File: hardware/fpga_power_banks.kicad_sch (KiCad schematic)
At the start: 0 parts

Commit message: update FPGA banks schematics
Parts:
- added U4: MPFS025T-FCVG484E, MPFS250T/MPFS160T/MPFS095T/MPFS025T-FCVG484_MCH, symbol payload-sym:MPFS025T-FCVG484E

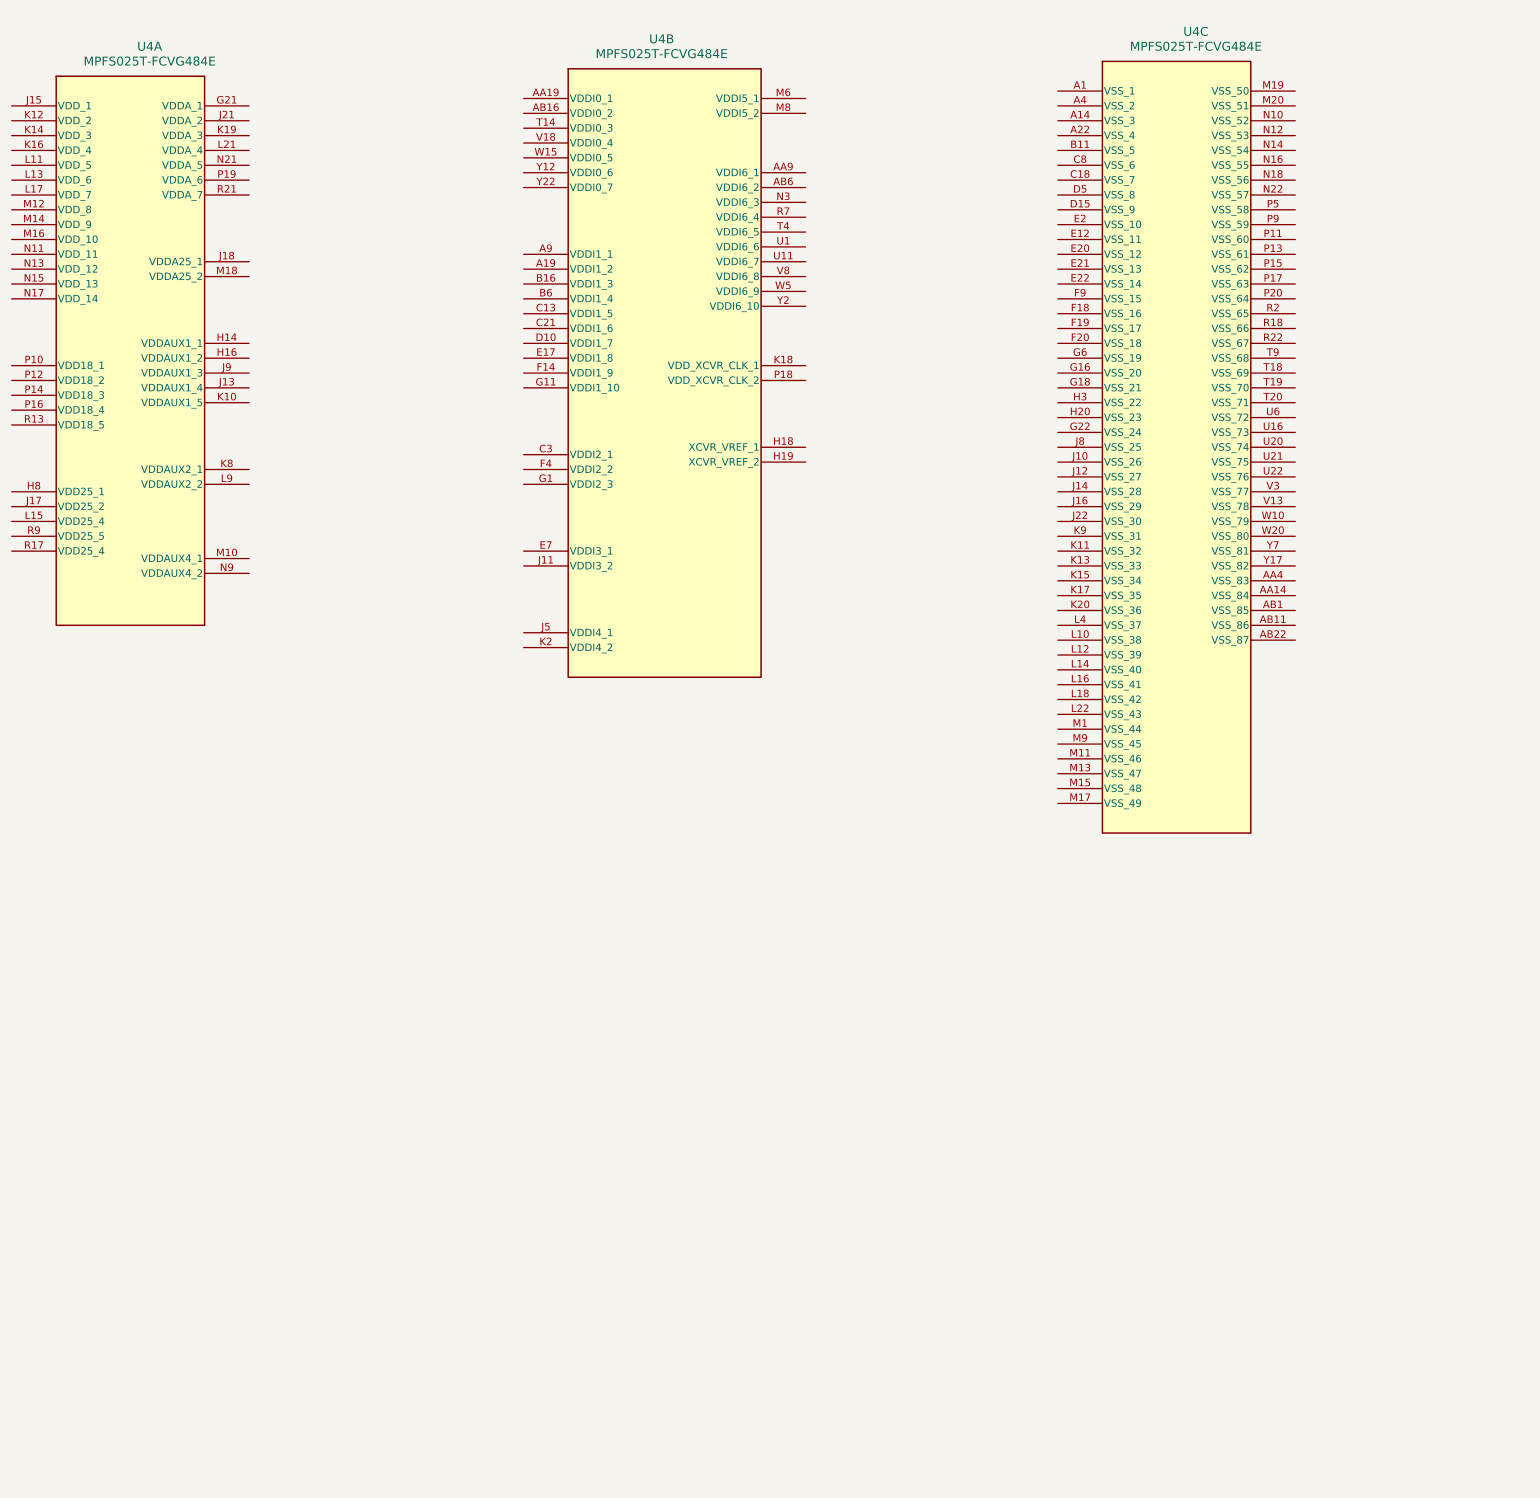
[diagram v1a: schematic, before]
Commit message: updated schematic
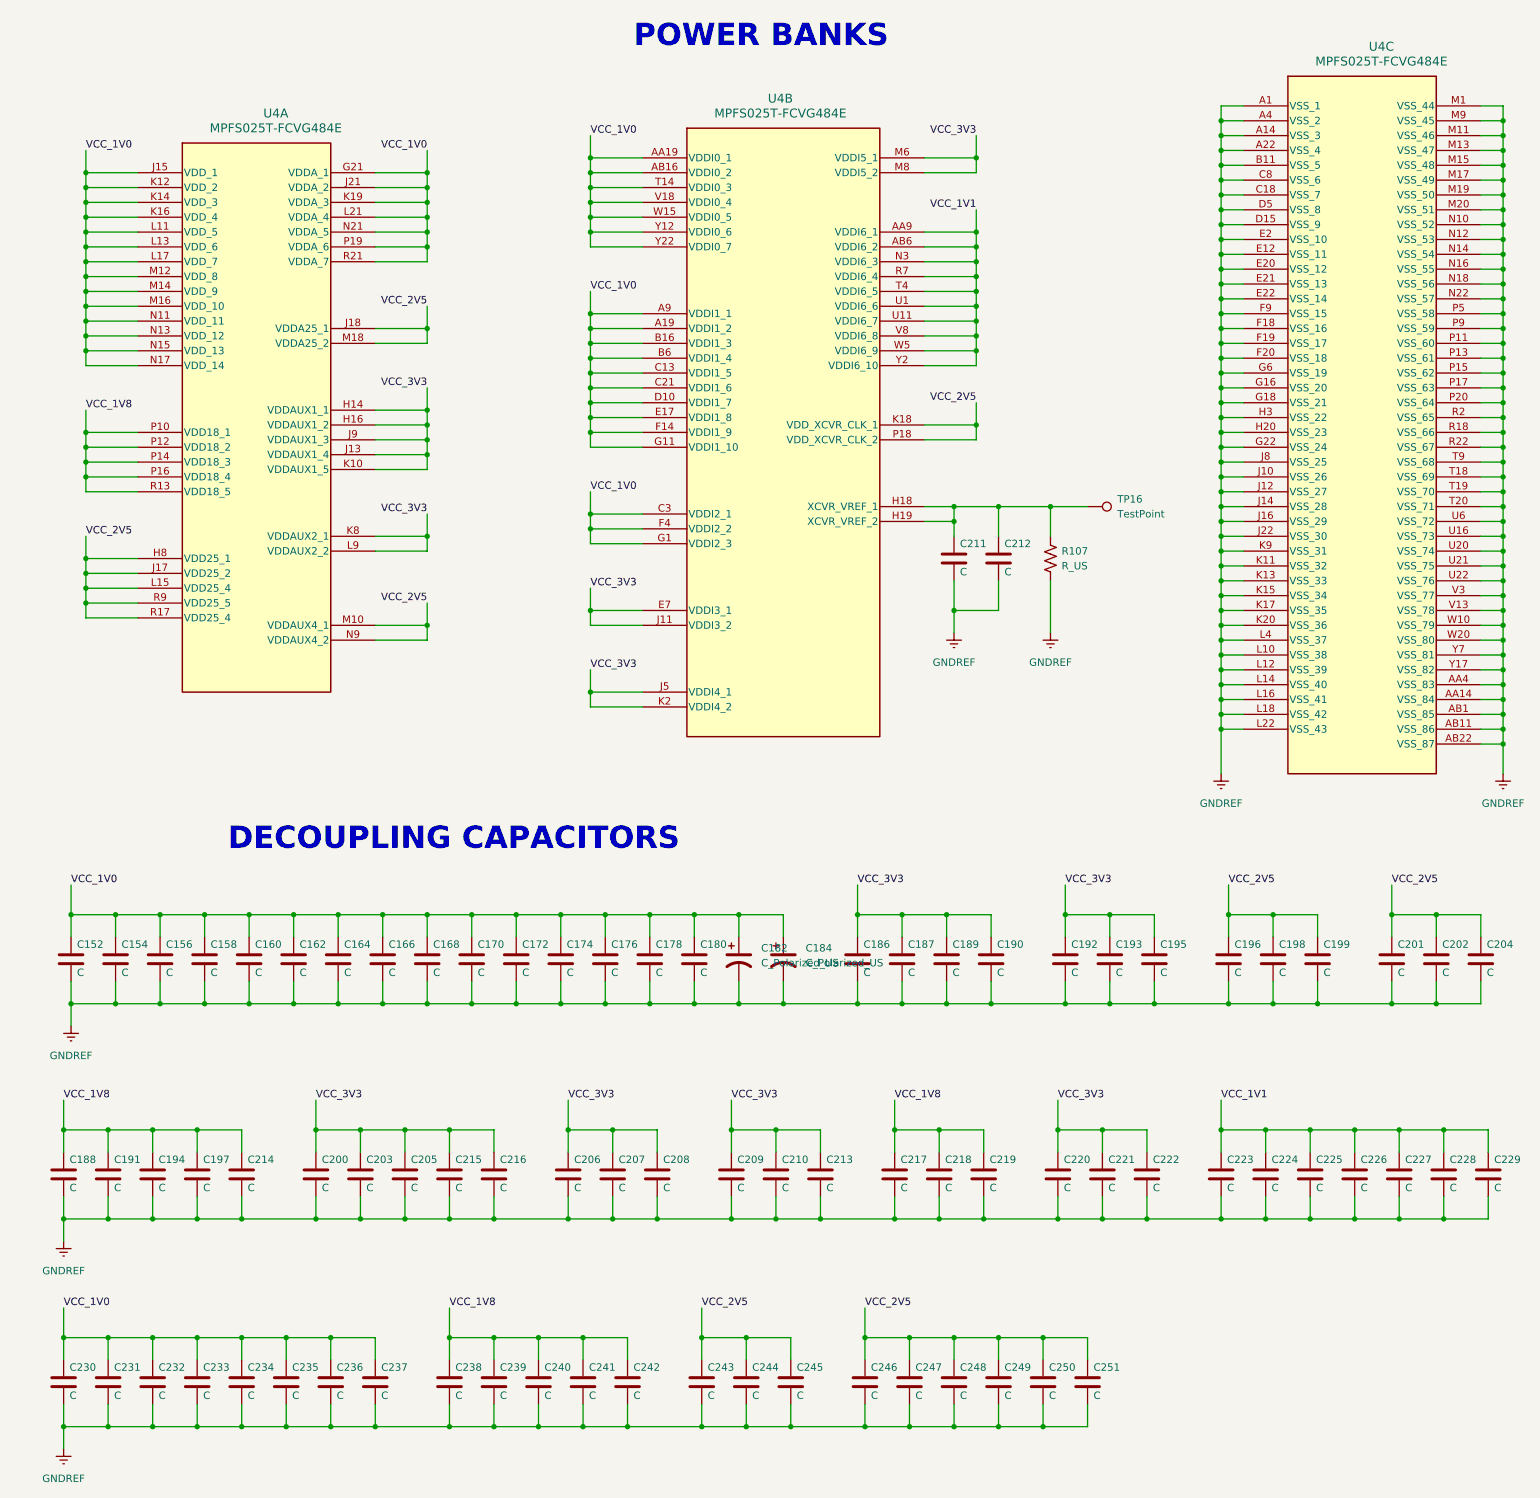
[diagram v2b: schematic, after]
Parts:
- added C152, C154, C156, C158, C160, C162, C164, C166, C168, C170, C172, C174, C176, C178, C180, C186, C187, C188, C189, C190, C191, C192, C193, C194, C195, C196, C197, C198, C199, C200, C201, C202, C203, C204, C205, C206, C207, C208, C209, C210, C211, C212, C213, C214, C215, C216, C217, C218, C219, C220, C221, C222, C223, C224, C225, C226, C227, C228, C229, C230, C231, C232, C233, C234, C235, C236, C237, C238, C239, C240, C241, C242, C243, C244, C245, C246, C247, C248, C249, C250, C251: C, symbol Device:C
- added C182, C184: C_Polarized_US, symbol Device:C_Polarized_US
- added R107: R_US, symbol Device:R_US
- added TP16: TestPoint, symbol Connector:TestPoint
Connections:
- net GNDREF: now reaches U4.A1 (VSS_1)
- net GNDREF: now also U4.A14 (VSS_3), U4.A22 (VSS_4), U4.A4 (VSS_2), U4.AA14 (VSS_84), U4.AA4 (VSS_83), U4.AB1 (VSS_85), U4.AB11 (VSS_86), U4.AB22 (VSS_87), U4.B11 (VSS_5), U4.C18 (VSS_7), U4.C8 (VSS_6), U4.D15 (VSS_9), U4.D5 (VSS_8), U4.E12 (VSS_11), U4.E2 (VSS_10), U4.E20 (VSS_12), U4.E21 (VSS_13), U4.E22 (VSS_14), U4.F18 (VSS_16), U4.F19 (VSS_17), U4.F20 (VSS_18), U4.F9 (VSS_15), U4.G16 (VSS_20), U4.G18 (VSS_21), U4.G22 (VSS_24), U4.G6 (VSS_19), U4.H20 (VSS_23), U4.H3 (VSS_22), U4.J10 (VSS_26), U4.J12 (VSS_27), U4.J14 (VSS_28), U4.J16 (VSS_29), U4.J22 (VSS_30), U4.J8 (VSS_25), U4.K11 (VSS_32), U4.K13 (VSS_33), U4.K15 (VSS_34), U4.K17 (VSS_35), U4.K20 (VSS_36), U4.K9 (VSS_31), U4.L10 (VSS_38), U4.L12 (VSS_39), U4.L14 (VSS_40), U4.L16 (VSS_41), U4.L18 (VSS_42), U4.L22 (VSS_43), U4.L4 (VSS_37), U4.M1 (VSS_44), U4.M11 (VSS_46), U4.M13 (VSS_47), U4.M15 (VSS_48), U4.M17 (VSS_49), U4.M19 (VSS_50), U4.M20 (VSS_51), U4.M9 (VSS_45), U4.N10 (VSS_52), U4.N12 (VSS_53), U4.N14 (VSS_54), U4.N16 (VSS_55), U4.N18 (VSS_56), U4.N22 (VSS_57), U4.P11 (VSS_60), U4.P13 (VSS_61), U4.P15 (VSS_62), U4.P17 (VSS_63), U4.P20 (VSS_64), U4.P5 (VSS_58), U4.P9 (VSS_59), U4.R18 (VSS_66), U4.R2 (VSS_65), U4.R22 (VSS_67), U4.T18 (VSS_69), U4.T19 (VSS_70), U4.T20 (VSS_71), U4.T9 (VSS_68), U4.U16 (VSS_73), U4.U20 (VSS_74), U4.U21 (VSS_75), U4.U22 (VSS_76), U4.U6 (VSS_72), U4.V13 (VSS_78), U4.V3 (VSS_77), U4.W10 (VSS_79), U4.W20 (VSS_80), U4.Y17 (VSS_82), U4.Y7 (VSS_81), C152.1, C154.1, C156.1, C158.1, C160.1, C162.1, C164.1, C166.1, C168.1, C170.1, C172.1, C174.1, C176.1, C178.1, C180.1, C182.2, C184.2, C186.1, C187.1, C188.1, C189.1, C190.1, C191.1, C192.1, C193.1, C194.1, C195.1, C196.1, C197.1, C198.1, C199.1, C200.1, C201.1, C202.1, C203.1, C204.1, C205.1, C206.1, C207.1, C208.1, C209.1, C210.1, C211.1, C212.1, C213.1, C214.1, C215.1, C216.1, C217.1, C218.1, C219.1, C220.1, C221.1, C222.1, C223.1, C224.1, C225.1, C226.1, C227.1, C228.1, C229.1, C230.1, C231.1, C232.1, C233.1, C234.1, C235.1, C236.1, C237.1, C238.1, C239.1, C240.1, C241.1, C242.1, C243.1, C244.1, C245.1, C246.1, C247.1, C248.1, C249.1, C250.1, C251.1, R107.1
- net VCC_1V0: now reaches U4.A19 (VDDI1_2)
- net VCC_1V0: now also U4.A9 (VDDI1_1), U4.AA19 (VDDI0_1), U4.AB16 (VDDI0_2), U4.B16 (VDDI1_3), U4.B6 (VDDI1_4), U4.C13 (VDDI1_5), U4.C21 (VDDI1_6), U4.C3 (VDDI2_1), U4.D10 (VDDI1_7), U4.E17 (VDDI1_8), U4.F14 (VDDI1_9), U4.F4 (VDDI2_2), U4.G1 (VDDI2_3), U4.G11 (VDDI1_10), U4.G21 (VDDA_1), U4.J15 (VDD_1), U4.J21 (VDDA_2), U4.K12 (VDD_2), U4.K14 (VDD_3), U4.K16 (VDD_4), U4.K19 (VDDA_3), U4.L11 (VDD_5), U4.L13 (VDD_6), U4.L17 (VDD_7), U4.L21 (VDDA_4), U4.M12 (VDD_8), U4.M14 (VDD_9), U4.M16 (VDD_10), U4.N11 (VDD_11), U4.N13 (VDD_12), U4.N15 (VDD_13), U4.N17 (VDD_14), U4.N21 (VDDA_5), U4.P19 (VDDA_6), U4.R21 (VDDA_7), U4.T14 (VDDI0_3), U4.V18 (VDDI0_4), U4.W15 (VDDI0_5), U4.Y12 (VDDI0_6), U4.Y22 (VDDI0_7), C152.2, C154.2, C156.2, C158.2, C160.2, C162.2, C164.2, C166.2, C168.2, C170.2, C172.2, C174.2, C176.2, C178.2, C180.2, C182.1, C184.1, C230.2, C231.2, C232.2, C233.2, C234.2, C235.2, C236.2, C237.2
- net VCC_1V1: now reaches U4.AA9 (VDDI6_1)
- net VCC_1V1: now also U4.AB6 (VDDI6_2), U4.N3 (VDDI6_3), U4.R7 (VDDI6_4), U4.T4 (VDDI6_5), U4.U1 (VDDI6_6), U4.U11 (VDDI6_7), U4.V8 (VDDI6_8), U4.W5 (VDDI6_9), U4.Y2 (VDDI6_10), C223.2, C224.2, C225.2, C226.2, C227.2, C228.2, C229.2
- net VCC_3V3: now reaches U4.E7 (VDDI3_1)
- net VCC_3V3: now also U4.H14 (VDDAUX1_1), U4.H16 (VDDAUX1_2), U4.J11 (VDDI3_2), U4.J13 (VDDAUX1_4), U4.J5 (VDDI4_1), U4.J9 (VDDAUX1_3), U4.K10 (VDDAUX1_5), U4.K2 (VDDI4_2), U4.K8 (VDDAUX2_1), U4.L9 (VDDAUX2_2), U4.M6 (VDDI5_1), U4.M8 (VDDI5_2), C186.2, C187.2, C189.2, C190.2, C192.2, C193.2, C195.2, C200.2, C203.2, C205.2, C206.2, C207.2, C208.2, C209.2, C210.2, C213.2, C215.2, C216.2, C220.2, C221.2, C222.2
- net at U4.H18 (XCVR_VREF_1): now also U4.H19 (XCVR_VREF_2), C211.2, C212.2, R107.2, TP16.1
- net VCC_2V5: now reaches U4.K18 (VDD_XCVR_CLK_1)
- net VCC_2V5: now also U4.H8 (VDD25_1), U4.J17 (VDD25_2), U4.J18 (VDDA25_1), U4.L15 (VDD25_4), U4.M10 (VDDAUX4_1), U4.M18 (VDDA25_2), U4.N9 (VDDAUX4_2), U4.P18 (VDD_XCVR_CLK_2), U4.R17 (VDD25_4), U4.R9 (VDD25_5), C196.2, C198.2, C199.2, C201.2, C202.2, C204.2, C243.2, C244.2, C245.2, C246.2, C247.2, C248.2, C249.2, C250.2, C251.2
- net VCC_1V8: now reaches U4.P10 (VDD18_1)
- net VCC_1V8: now also U4.P12 (VDD18_2), U4.P14 (VDD18_3), U4.P16 (VDD18_4), U4.R13 (VDD18_5), C188.2, C191.2, C194.2, C197.2, C214.2, C217.2, C218.2, C219.2, C238.2, C239.2, C240.2, C241.2, C242.2
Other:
- note added: "DECOUPLING CAPACITORS"
- note added: "POWER BANKS"
- moved on the sheet: U4A, U4B, U4C
